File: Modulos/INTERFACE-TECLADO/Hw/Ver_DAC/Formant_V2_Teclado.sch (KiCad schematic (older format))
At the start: 85 parts

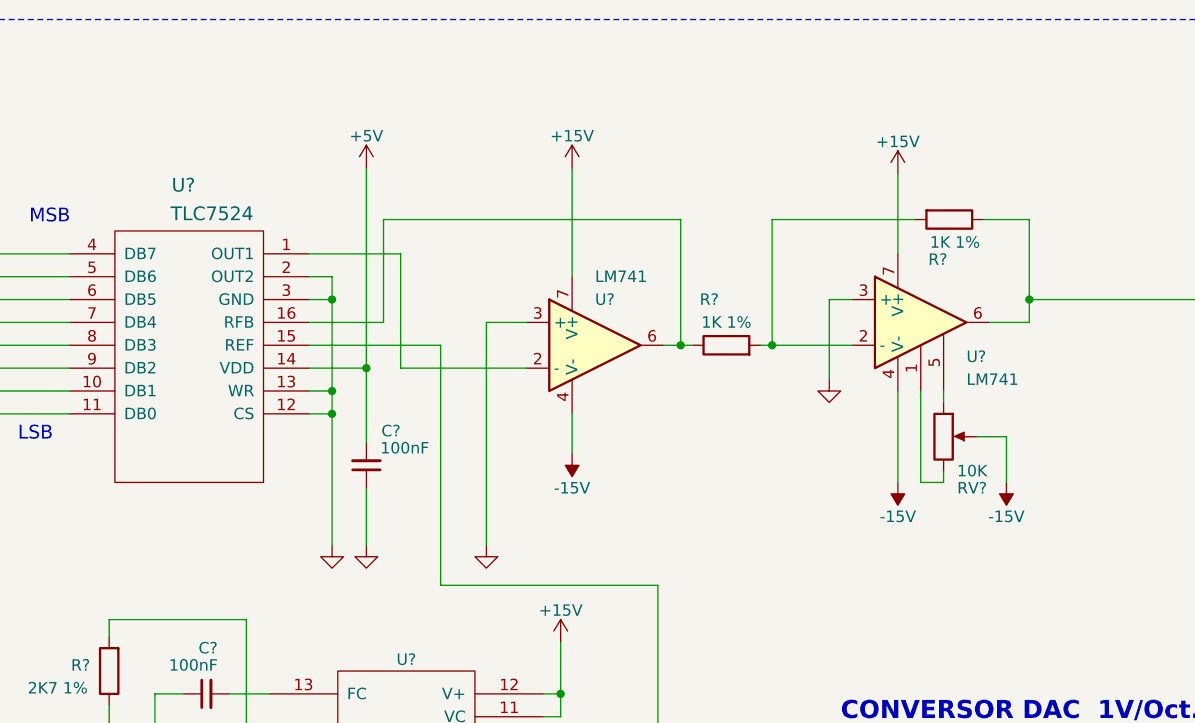
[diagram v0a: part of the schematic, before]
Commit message: Actualizacion Interfaz Teclado
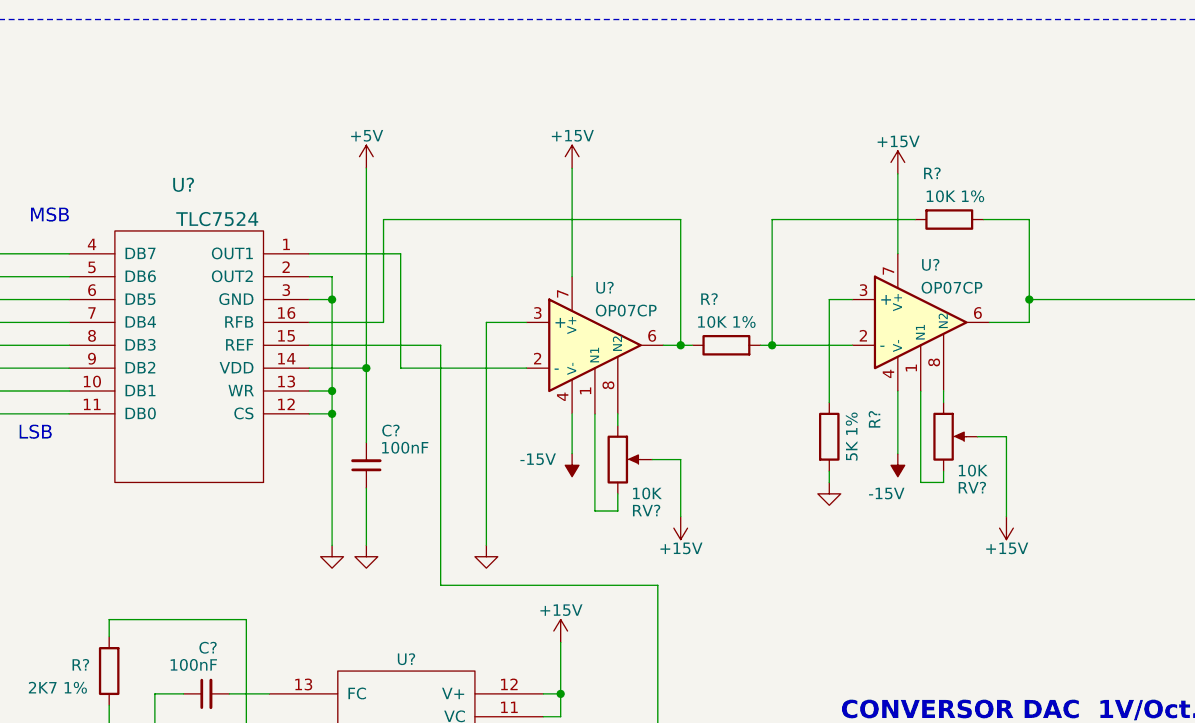
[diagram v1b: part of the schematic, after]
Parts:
- removed U?: LM741, symbol TL071
- removed U?: LM741, symbol LM741
- removed U?: TLC7524, symbol TLC7524
- added R?: 5K 1%, symbol R
- added RV?: 10K, symbol POT
- added U?: TLC7524, symbol TLC7524
- added U? (x2): OP07CP, symbol OP07CP
- R? (x2): value 1K 1% -> 10K 1%
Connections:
- net +15V: now also RV?.2, RV?.2, U?.7 (V+), U?.7 (V+)
- net +5V: now also U?.14 (VDD)
- net -15V: now also U?.4 (V-), U?.4 (V-); no longer RV?.2
- net GND: now also R?.2, U?.12 (CS), U?.13 (WR), U?.2 (OUT2), U?.3 (+), U?.3 (GND)
- net KBV: now also U?.6
- net TECLADO_D0: now also U?.11 (DB0)
- net TECLADO_D1: now also U?.10 (DB1)
- net TECLADO_D2: now also U?.9 (DB2)
- net TECLADO_D3: now also U?.8 (DB3)
- net TECLADO_D4: now also U?.7 (DB4)
- net TECLADO_D5: now also U?.6 (DB5)
- net TECLADO_D6: now also U?.5 (DB6)
- net TECLADO_D7: now also U?.4 (DB7)
- net at R?.1: now also U?.16 (RFB), U?.6
- net at R?.2, R?.2: now also U?.2 (-)
- net at RV?.3: now also U?.1 (N1)
- net at RV?.1: now also U?.8 (N2)
- net at R?.1, R?.2, U?.3 (SEN): now also U?.15 (REF)
- new net: U?.1 (OUT1), U?.2 (-)
- new net: RV?.3, U?.1 (N1)
- new net: RV?.1, U?.8 (N2)
- new net: R?.1, U?.3 (+)
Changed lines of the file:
@@
 EESchema Schematic File Version 2
+LIBS:Formant_V2_Teclado-rescue
 LIBS:power
 LIBS:device
@@
 Wire Wire Line
 	7300 7850 7300 7925
-$Comp
-L TL071 U?
-U 1 1 5A2BB558
-P 4375 2100
-F 0 "U?" H 4375 2300 50  0000 L CNN
-F 1 "LM741" H 4375 2400 50  0000 L CNN
-F 2 "" H 4425 2300 50  0000 C CNN
-F 3 "" H 4375 2350 50  0000 C CNN
-	1    4375 2100
-	1    0    0    -1
-$EndComp
 Wire Wire Line
 	3525 2200 4075 2200
@@
 P 4275 2575
 F 0 "#PWR?" H 4275 2675 50  0001 C CNN
-F 1 "-15V" H 4275 2725 50  0000 C CNN
+F 1 "-15V" H 4425 2600 50  0000 C CNN
 F 2 "" H 4275 2575 50  0000 C CNN
 F 3 "" H 4275 2575 50  0000 C CNN
@@
 P 4950 2100
 F 0 "R?" V 5150 2175 50  0000 C CNN
-F 1 "1K 1%" V 5050 2100 50  0000 C CNN
+F 1 "10K 1%" V 5050 2100 50  0000 C CNN
 F 2 "" V 4880 2100 50  0000 C CNN
 F 3 "" H 4950 2100 50  0000 C CNN
@@
 	1    0    0    -1
 $EndComp
-Wire Wire Line
-	5700 2300 5700 2700
 $Comp
 L -15V #PWR?
 U 1 1 5A2BB56F
-P 5700 2700
-F 0 "#PWR?" H 5700 2800 50  0001 C CNN
-F 1 "-15V" H 5700 2850 50  0000 C CNN
-F 2 "" H 5700 2700 50  0000 C CNN
-F 3 "" H 5700 2700 50  0000 C CNN
-	1    5700 2700
+P 5700 2575
+F 0 "#PWR?" H 5700 2675 50  0001 C CNN
+F 1 "-15V" H 5750 2750 50  0000 C CNN
+F 2 "" H 5700 2575 50  0000 C CNN
+F 3 "" H 5700 2575 50  0000 C CNN
+	1    5700 2575
 	-1   0    0    1
 $EndComp
@@
 U 1 1 5A2BB570
 P 5925 1550
-F 0 "R?" V 6100 1500 50  0000 C CNN
-F 1 "1K 1%" V 6025 1575 50  0000 C CNN
+F 0 "R?" V 5725 1475 50  0000 C CNN
+F 1 "10K 1%" V 5825 1575 50  0000 C CNN
 F 2 "" V 5855 1550 50  0000 C CNN
 F 3 "" H 5925 1550 50  0000 C CNN
@@
 Wire Wire Line
 	2075 2400 1350 2400
-$Comp
-L LM741 U?
-U 1 1 5A2BB573
-P 5800 2000
-F 0 "U?" H 6000 1850 50  0000 L CNN
-F 1 "LM741" H 6000 1750 50  0000 L CNN
-F 2 "" H 5850 2050 50  0000 C CNN
-F 3 "" H 5950 2150 50  0000 C CNN
-	1    5800 2000
-	1    0    0    -1
-$EndComp
 Wire Wire Line
 	5100 2100 5500 2100
@@
 Wire Wire Line
 	5800 2700 5800 2300
-$Comp
-L -15V #PWR?
-U 1 1 5A2BB577
-P 6175 2700
-F 0 "#PWR?" H 6175 2800 50  0001 C CNN
-F 1 "-15V" H 6175 2850 50  0000 C CNN
-F 2 "" H 6175 2700 50  0000 C CNN
-F 3 "" H 6175 2700 50  0000 C CNN
-	1    6175 2700
-	-1   0    0    1
-$EndComp
 Wire Wire Line
 	6050 2500 6175 2500
 Wire Wire Line
-	6175 2500 6175 2700
+	6175 2500 6175 2850
 Text GLabel 7375 1900 2    60   Output ~ 0
 KBV
@@
 	7375 1900 6275 1900
 Connection ~ 6275 1900
-$Comp
-L TLC7524 U?
-U 1 1 5A3049AD
-P 2475 1450
-F 0 "U?" H 2575 1500 60  0000 C CNN
-F 1 "TLC7524" H 2700 1375 60  0000 C CNN
-F 2 "" H 2475 1450 60  0001 C CNN
-F 3 "" H 2475 1450 60  0001 C CNN
-	1    2475 1450
-	1    0    0    -1
-$EndComp
 Wire Wire Line
 	3125 2300 3225 2300
@@
 L GND #PWR?
 U 1 1 5A311945
-P 5400 2250
-F 0 "#PWR?" H 5400 2000 50  0001 C CNN
-F 1 "GND" H 5400 2100 50  0001 C CNN
-F 2 "" H 5400 2250 50  0000 C CNN
-F 3 "" H 5400 2250 50  0000 C CNN
-	1    5400 2250
+P 5400 2700
+F 0 "#PWR?" H 5400 2450 50  0001 C CNN
+F 1 "GND" H 5400 2550 50  0001 C CNN
+F 2 "" H 5400 2700 50  0000 C CNN
+F 3 "" H 5400 2700 50  0000 C CNN
+	1    5400 2700
 	1    0    0    -1
 $EndComp
 Wire Wire Line
 	5500 1900 5400 1900
-Wire Wire Line
-	5400 1900 5400 2250
+$Comp
+L TLC7524 U?
+U 1 1 5A42C0B5
+P 2475 1450
+F 0 "U?" H 2575 1500 60  0000 C CNN
+F 1 "TLC7524" H 2725 1350 60  0000 C CNN
+F 2 "" H 2475 1450 60  0001 C CNN
+F 3 "" H 2475 1450 60  0001 C CNN
+	1    2475 1450
+	1    0    0    -1
+$EndComp
+$Comp
+L OP07CP U?
+U 1 1 5A42C470
+P 4375 2100
+F 0 "U?" H 4375 2350 50  0000 L CNN
+F 1 "OP07CP" H 4375 2250 50  0000 L CNN
+F 2 "" H 4425 2150 50  0000 C CNN
+F 3 "" H 4525 2250 50  0000 C CNN
+	1    4375 2100
+	1    0    0    -1
+$EndComp
+$Comp
+L OP07CP U?
+U 1 1 5A42C7C7
+P 5800 2000
+F 0 "U?" H 5800 2250 50  0000 L CNN
+F 1 "OP07CP" H 5800 2150 50  0000 L CNN
+F 2 "" H 5850 2050 50  0000 C CNN
+F 3 "" H 5950 2150 50  0000 C CNN
+	1    5800 2000
+	1    0    0    -1
+$EndComp
+$Comp
+L R R?
+U 1 1 5A42D375
+P 5400 2500
+F 0 "R?" V 5600 2575 50  0000 C CNN
+F 1 "5K 1%" V 5500 2500 50  0000 C CNN
+F 2 "" V 5330 2500 50  0000 C CNN
+F 3 "" H 5400 2500 50  0000 C CNN
+	1    5400 2500
+	1    0    0    -1
+$EndComp
+Wire Wire Line
+	5400 1900 5400 2350
+Wire Wire Line
+	5400 2650 5400 2700
+$Comp
+L POT RV?
+U 1 1 5A42DDFB
+P 4475 2600
+F 0 "RV?" H 4600 2375 50  0000 C CNN
+F 1 "10K" H 4600 2450 50  0000 C CNN
+F 2 "" H 4475 2600 50  0000 C CNN
+F 3 "" H 4475 2600 50  0000 C CNN
+	1    4475 2600
+	1    0    0    -1
+$EndComp
+$Comp
+L +15V #PWR?
+U 1 1 5A42E12C
+P 6175 2850
+F 0 "#PWR?" H 6175 2700 50  0001 C CNN
+F 1 "+15V" H 6175 2990 50  0000 C CNN
+F 2 "" H 6175 2850 50  0000 C CNN
+F 3 "" H 6175 2850 50  0000 C CNN
+	1    6175 2850
+	-1   0    0    1
+$EndComp
+Wire Wire Line
+	4475 2400 4475 2450
+Wire Wire Line
+	4375 2400 4375 2825
+Wire Wire Line
+	4375 2825 4475 2825
+Wire Wire Line
+	4475 2825 4475 2750
+Wire Wire Line
+	5700 2300 5700 2575
+$Comp
+L +15V #PWR?
+U 1 1 5A42EE59
+P 4750 2850
+F 0 "#PWR?" H 4750 2700 50  0001 C CNN
+F 1 "+15V" H 4750 2990 50  0000 C CNN
+F 2 "" H 4750 2850 50  0000 C CNN
+F 3 "" H 4750 2850 50  0000 C CNN
+	1    4750 2850
+	-1   0    0    1
+$EndComp
+Wire Wire Line
+	4625 2600 4750 2600
+Wire Wire Line
+	4750 2600 4750 2850
 $EndSCHEMATC
